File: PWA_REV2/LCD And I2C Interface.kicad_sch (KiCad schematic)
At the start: 44 parts, among them Q301 BSS138, Q401 BSS138, Q402 BSS138, U301 PCF8574AT_3_518, U302 LCD_20x4_Character-GPAD_SCH_L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, U303 Conn_01x16

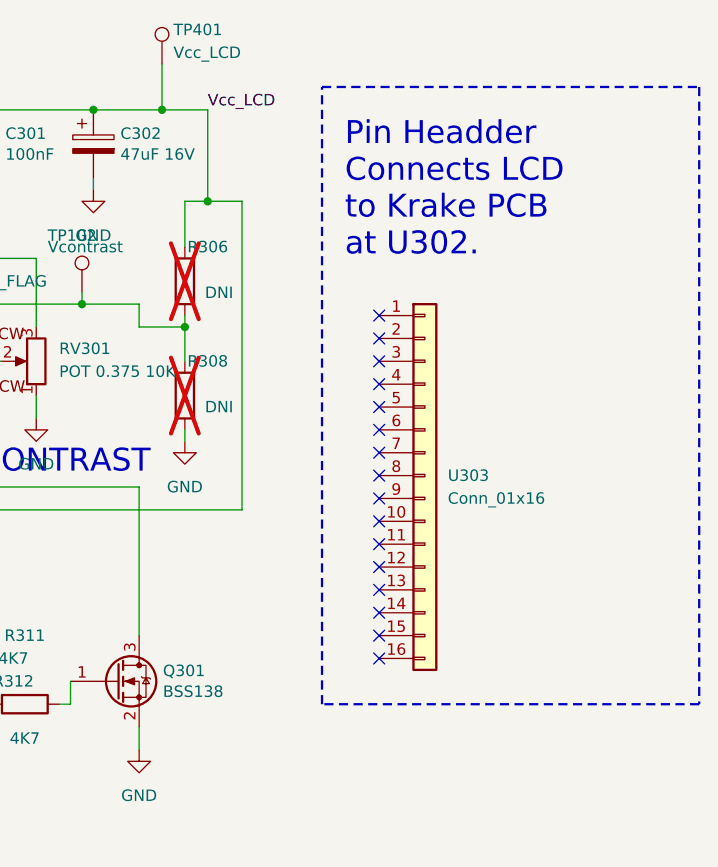
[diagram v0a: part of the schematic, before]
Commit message: fixed kicad project issue.
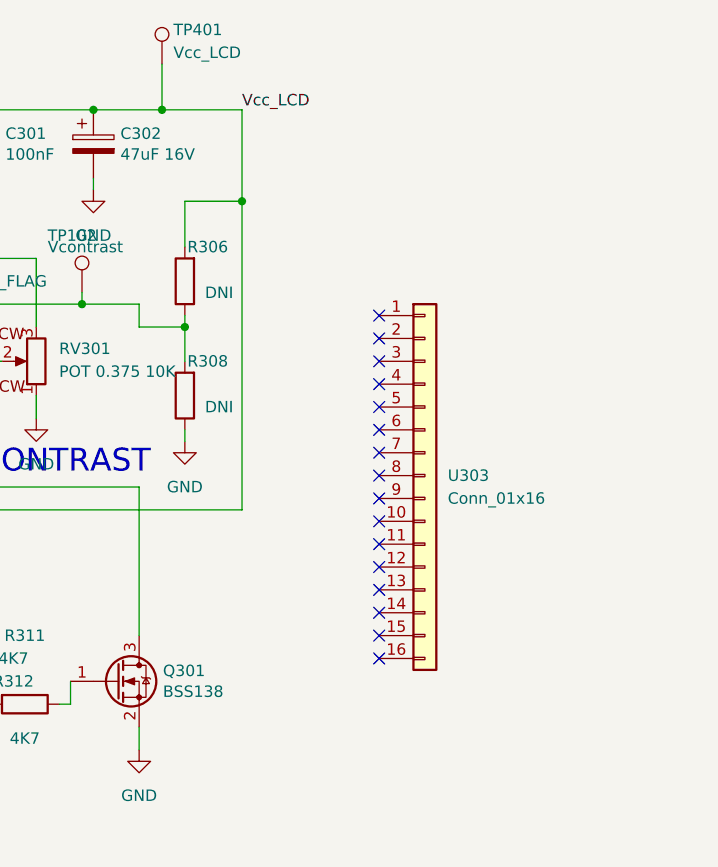
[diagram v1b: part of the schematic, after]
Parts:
- R306, R308: now fitted
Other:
- note removed: "Pin Headder Connects LCD to Krake PCB at U302."
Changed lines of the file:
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@@
   (junction (at 173.99 77.47) (diameter 0) (color 0 0 0 0)
   )
+  (junction (at 232.41 50.8) (diameter 0) (color 0 0 0 0)
+  )
   (junction (at 69.85 77.47) (diameter 0) (color 0 0 0 0)
   )
@@
   )
   (junction (at 116.84 52.07) (diameter 0) (color 0 0 0 0)
-  )
-  (junction (at 228.6 50.8) (diameter 0) (color 0 0 0 0)
   )
   (junction (at 198.12 62.23) (diameter 0) (color 0 0 0 0)
@@
     (stroke (width 0) (type default))
   )
-  (wire (pts (xy 228.6 50.8) (xy 232.41 50.8))
-    (stroke (width 0) (type default))
-  )
   (wire (pts (xy 195.58 66.04) (xy 196.85 66.04))
     (stroke (width 0) (type default))
@@
     (stroke (width 0) (type default))
   )
-  (wire (pts (xy 223.52 40.64) (xy 228.6 40.64))
+  (wire (pts (xy 223.52 40.64) (xy 232.41 40.64))
     (stroke (width 0) (type default))
   )
@@
     (stroke (width 0) (type default))
   )
-  (wire (pts (xy 226.06 50.8) (xy 228.6 50.8))
+  (wire (pts (xy 226.06 50.8) (xy 232.41 50.8))
     (stroke (width 0) (type default))
   )
@@
     (stroke (width 0) (type default))
   )
-  (wire (pts (xy 228.6 40.64) (xy 228.6 50.8))
+  (wire (pts (xy 232.41 40.64) (xy 232.41 50.8))
     (stroke (width 0) (type default))
   )
@@
   (wire (pts (xy 40.64 53.34) (xy 53.34 53.34))
     (stroke (width 0) (type default))
-  )
-  (rectangle (start 241.3 38.1) (end 283.21 106.68)
-    (stroke (width 0.254) (type dash))
-    (fill (type none))
   )
   (image (at 124.46 137.16) (scale 1.35089)
@@
     )
   )
-  (text "Pin Headder\nConnects LCD\nto Krake PCB\nat U302." (at 243.84 57.15 0)
-    (effects (font (size 2.54 2.54)) (justify left bottom))
-  )
   (text "Wiring of I2C to LCD from:\nhttps://alselectro.wordpress.com/2016/05/12/serial-lcd-i2c-module-pcf8574/"
     (at 92.71 40.64 0)
@@
     (effects (font (size 1.524 1.524)) (justify left bottom))
   )
-  (label "Vcc_LCD" (at 228.6 40.64 0) (fields_autoplaced)
+  (label "Vcc_LCD" (at 232.41 40.64 0) (fields_autoplaced)
     (effects (font (size 1.27 1.27)) (justify left bottom))
   )
@@
   )
   (symbol (lib_id "Device:R") (at 226.06 59.69 180) (unit 1)
-    (in_bom yes) (on_board yes) (dnp yes)
+    (in_bom yes) (on_board yes) (dnp no)
     (property "Reference" "R306" (at 228.6 55.88 0)
       (effects (font (size 1.27 1.27)))
@@
   )
   (symbol (lib_id "Device:R") (at 226.06 72.39 180) (unit 1)
-    (in_bom yes) (on_board yes) (dnp yes)
+    (in_bom yes) (on_board yes) (dnp no)
     (property "Reference" "R308" (at 228.6 68.58 0)
       (effects (font (size 1.27 1.27)))

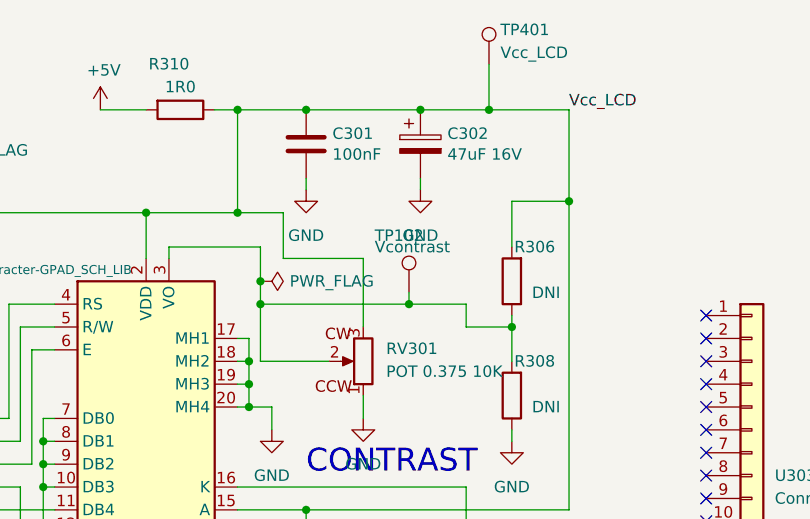
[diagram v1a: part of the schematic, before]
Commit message: Hardware, PWA, Add a Jumper to BOM for J102 so that USB Connector Can Power Krake, issue 312.
:q
q
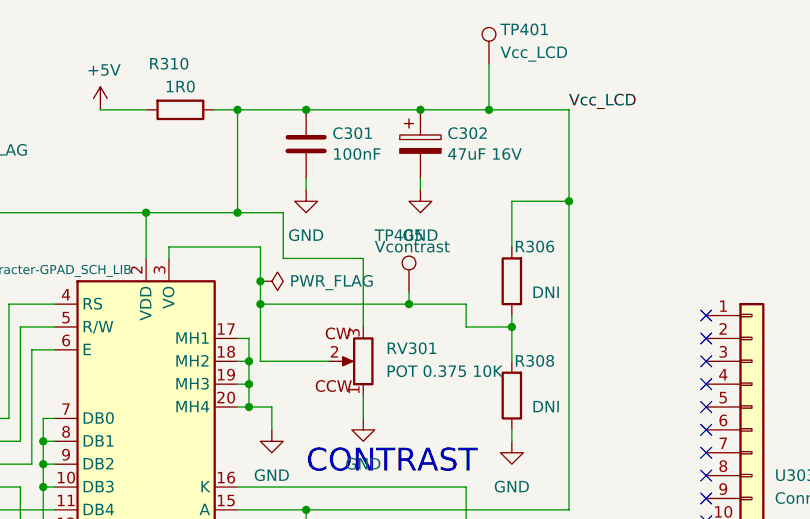
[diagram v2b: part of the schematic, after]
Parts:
- renumbered TP102 to TP405

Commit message: Revert "Hardware, PWA, Add a Jumper to BOM for J102 so that USB Connector Can Power Krake, issue 312."
This reverts commit c2819b8ee4999f733f52d823f88f6aefd6456fcc.
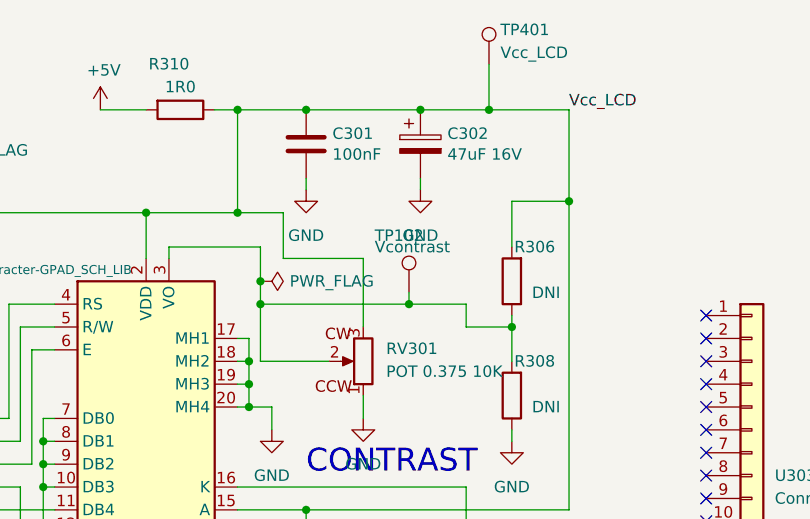
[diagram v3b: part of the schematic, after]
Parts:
- renumbered TP405 to TP102
